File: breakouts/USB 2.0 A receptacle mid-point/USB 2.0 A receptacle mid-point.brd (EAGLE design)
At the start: 21.3 x 31.8 mm, 3 parts

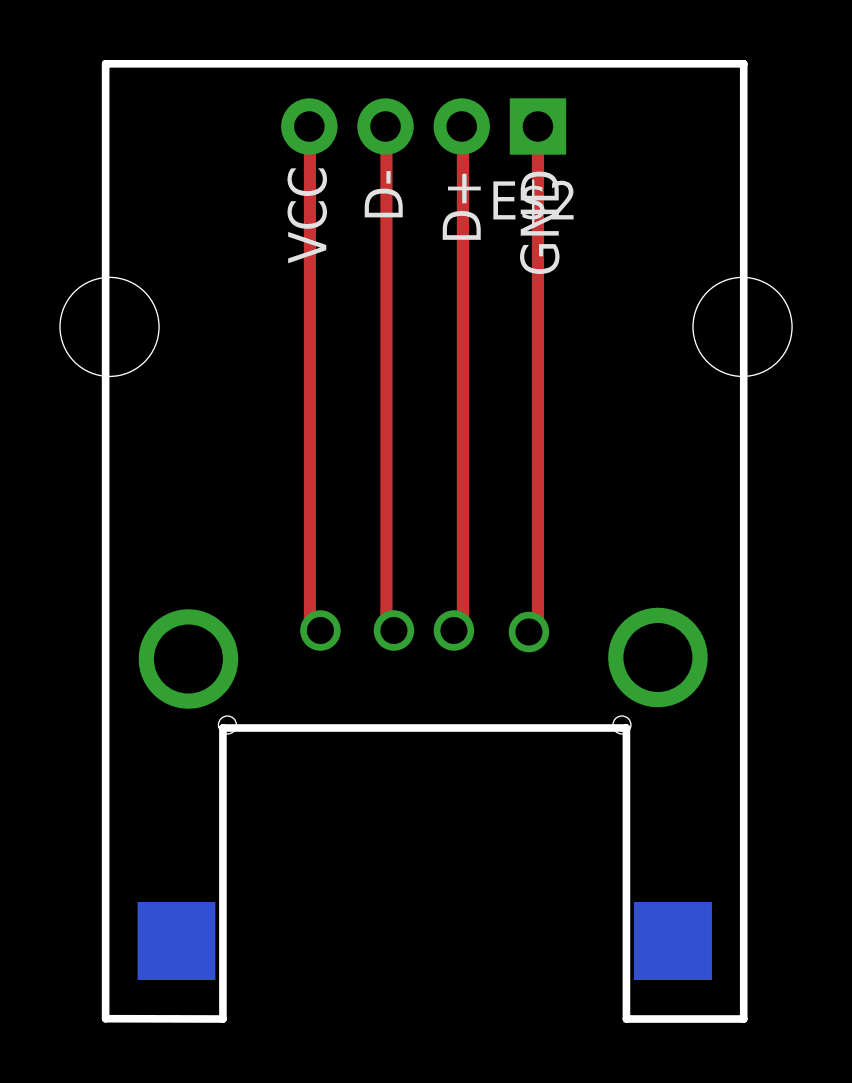
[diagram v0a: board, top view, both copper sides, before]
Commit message: a little too tight...
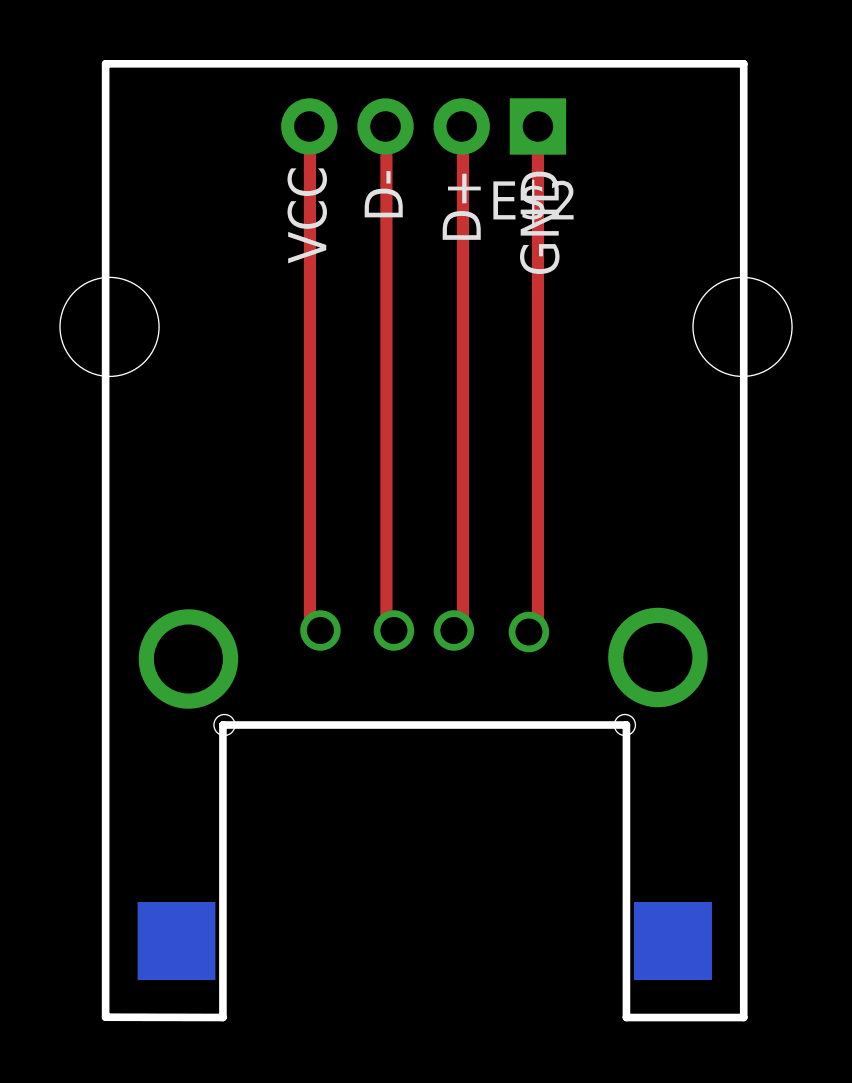
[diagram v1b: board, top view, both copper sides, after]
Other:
- outline, holes or cut-outs redrawn
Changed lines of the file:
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@@
 <board>
 <plain>
-<wire x1="12.29" y1="3.56" x2="12.29" y2="35.39" width="0.254" layer="20"/>
+<wire x1="12.29" y1="3.61" x2="12.29" y2="35.39" width="0.254" layer="20"/>
 <wire x1="12.29" y1="35.39" x2="33.56" y2="35.39" width="0.254" layer="20"/>
-<wire x1="33.56" y1="35.39" x2="33.56" y2="3.55" width="0.254" layer="20"/>
-<wire x1="33.56" y1="3.55" x2="29.65" y2="3.55" width="0.254" layer="20"/>
-<wire x1="29.65" y1="3.55" x2="29.65" y2="13.25" width="0.254" layer="20"/>
-<wire x1="29.65" y1="13.25" x2="16.2" y2="13.25" width="0.254" layer="20"/>
-<wire x1="16.2" y1="13.25" x2="16.2" y2="3.55" width="0.254" layer="20"/>
-<wire x1="16.2" y1="3.55" x2="12.29" y2="3.56" width="0.254" layer="20"/>
+<wire x1="33.56" y1="35.39" x2="33.56" y2="3.6" width="0.254" layer="20"/>
+<wire x1="33.56" y1="3.6" x2="29.65" y2="3.6" width="0.254" layer="20"/>
+<wire x1="29.65" y1="3.6" x2="29.65" y2="13.35" width="0.254" layer="20"/>
+<wire x1="29.65" y1="13.35" x2="16.2" y2="13.35" width="0.254" layer="20"/>
+<wire x1="16.2" y1="13.35" x2="16.2" y2="3.6" width="0.254" layer="20"/>
+<wire x1="16.2" y1="3.6" x2="12.29" y2="3.61" width="0.254" layer="20"/>
 <text x="26.125" y="31.89" size="1.27" layer="121" font="vector" ratio="15" rot="R270">GND</text>
 <text x="27.67" y="24.35" size="1.27" layer="122" font="vector" rot="MR0">quilix.com</text>
@@
 <dimension x1="12.29" y1="3.46" x2="12.3" y2="6.05" x3="6.941025" y3="4.775671875" layer="47"/>
 <dimension x1="29.65" y1="13.3" x2="32.7" y2="6.2" x3="41.95" y3="9.75" layer="47" dtype="vertical"/>
-<hole x="16.35" y="13.35" drill="0.6"/>
-<hole x="29.5" y="13.35" drill="0.6"/>
+<hole x="16.25" y="13.35" drill="0.7"/>
+<hole x="29.6" y="13.35" drill="0.7"/>
 <dimension x1="16.2" y1="3.55" x2="29.65" y2="3.55" x3="22.925" y3="-6.55" layer="47"/>
 <dimension x1="15.05" y1="15.55" x2="30.75" y2="15.55" x3="22.9" y3="22.2" layer="47"/>
@@
 <text x="20.925" y="31.89" size="1.27" layer="121" font="vector" ratio="15" rot="R270">D-</text>
 <text x="18.375" y="31.99" size="1.27" layer="121" font="vector" ratio="15" rot="R270">VCC</text>
+<rectangle x1="13.2" y1="4.7" x2="16.1" y2="7.6" layer="40"/>
+<rectangle x1="29.75" y1="4.75" x2="32.6" y2="7.55" layer="40"/>
 </plain>
 <attributes>
